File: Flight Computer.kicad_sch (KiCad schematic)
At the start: 28 parts, among them Q1 MMBT2222A, U6 STM32L476VETx, Y1 16MHz

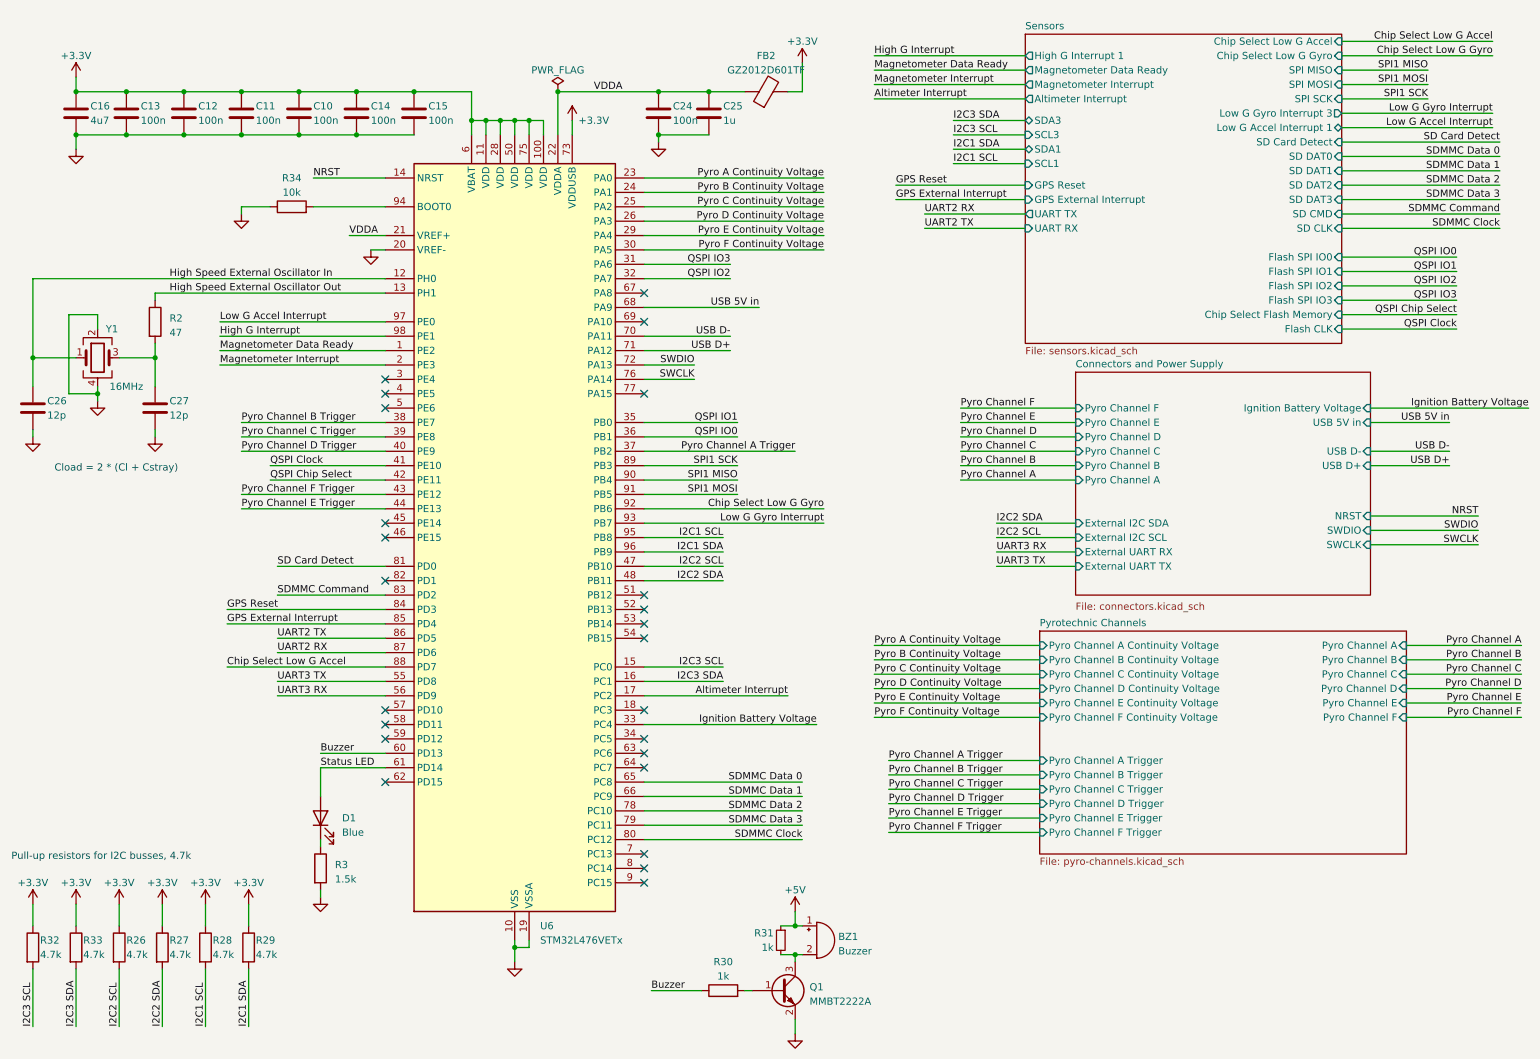
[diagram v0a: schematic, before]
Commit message: How many sheets do you want? Yes
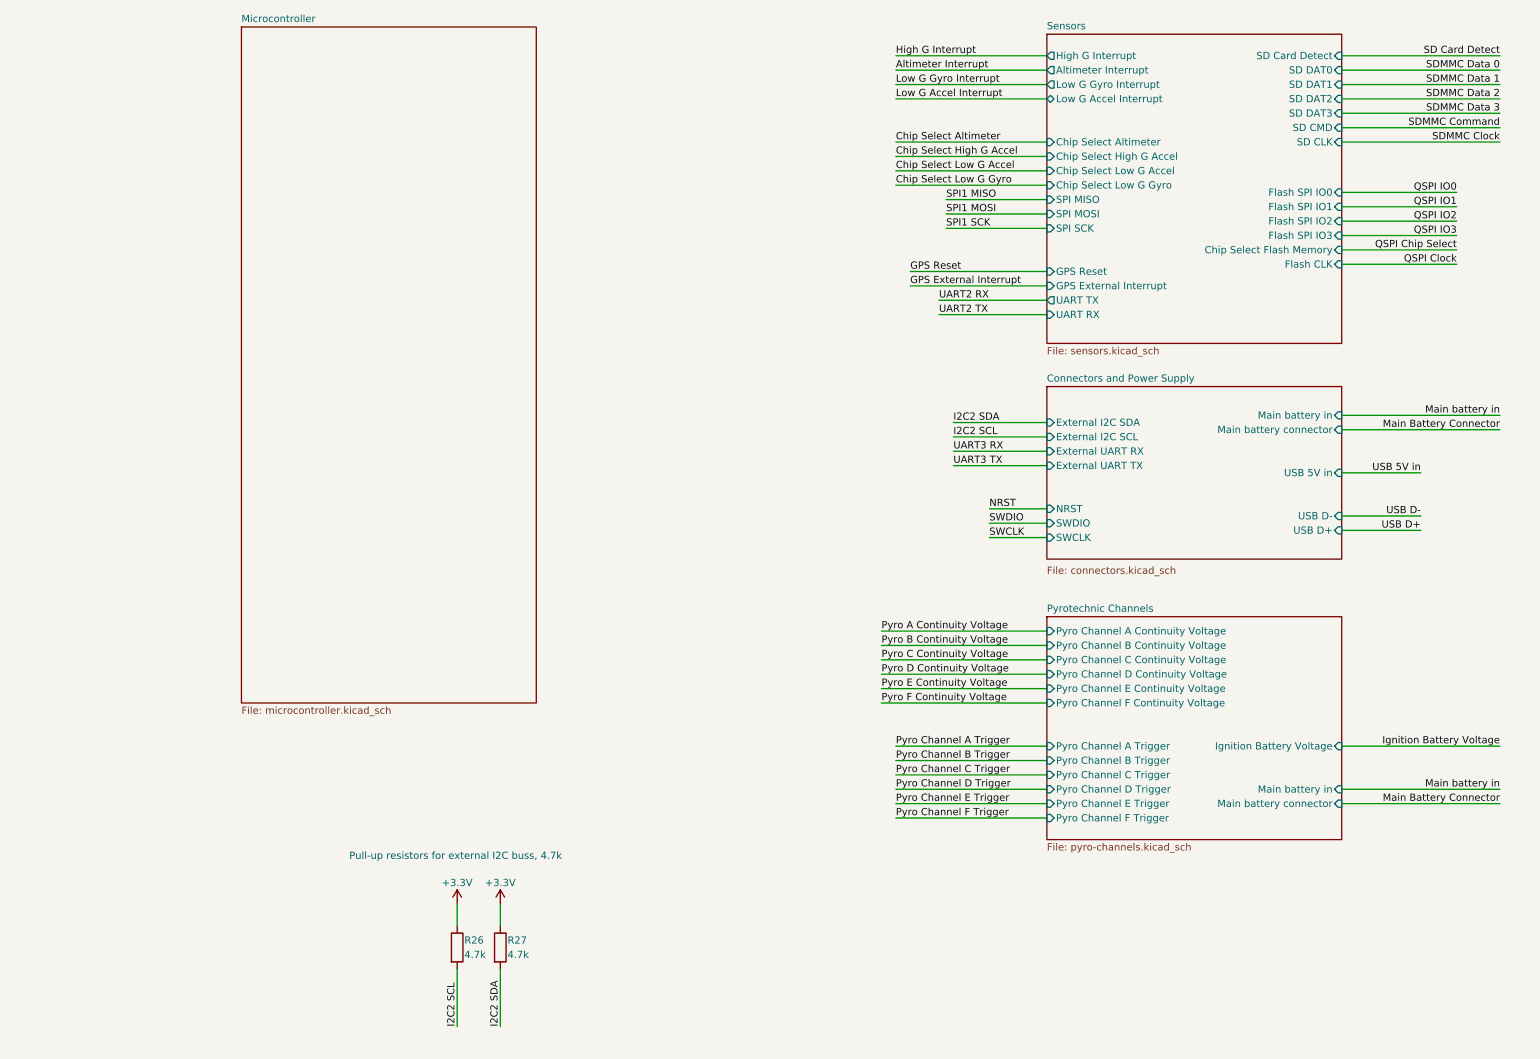
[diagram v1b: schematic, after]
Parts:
- removed BZ1: Buzzer, Buzzer_Beeper:Buzzer_TDK_PS1240P02BT_D12.2mm_H6.5mm, symbol Device:Buzzer
- removed C10, C11, C12, C13, C14, C15, C24: 100n, Capacitor_SMD:C_0402_1005Metric, symbol Device:C
- removed C16: 4u7, Capacitor_SMD:C_0603_1608Metric, symbol Device:C
- removed C25: 1u, Capacitor_SMD:C_0603_1608Metric, symbol Device:C
- removed C26, C27: 12p, Capacitor_SMD:C_0402_1005Metric, symbol Device:C
- removed D1: Blue, LED_SMD:LED_0805_2012Metric, symbol Device:LED
- removed FB2: GZ2012D601TF, Inductor_SMD:L_0805_2012Metric, symbol Device:FerriteBead
- removed Q1: MMBT2222A, Package_TO_SOT_SMD:SOT-23, symbol Transistor_BJT:MMBT3904
- removed R2: 47, Resistor_SMD:R_0603_1608Metric, symbol Device:R
- removed R28, R29, R32, R33: 4.7k, Resistor_SMD:R_0402_1005Metric, symbol Device:R
- removed R3: 1.5k, Resistor_SMD:R_0603_1608Metric, symbol Device:R
- removed R30: 1k, Resistor_SMD:R_0603_1608Metric, symbol Device:R
- removed R31: 1k, Resistor_SMD:R_0603_1608Metric, symbol Device:R_Small
- removed R34: 10k, Resistor_SMD:R_0402_1005Metric, symbol Device:R
- removed U6: STM32L476VETx, Package_QFP:LQFP-100_14x14mm_P0.5mm, symbol MCU_ST_STM32L4:STM32L476VETx
- removed Y1: 16MHz, Crystal:Crystal_SMD_3225-4Pin_3.2x2.5mm, symbol Device:Crystal_GND24
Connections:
- no-connect marks 24 -> 0
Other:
- added sheet Microcontroller (microcontroller.kicad_sch)
- sheet Connectors and Power Supply ports: added Main battery connector, Main battery in; removed Ignition Battery Voltage, Pyro Channel A, Pyro Channel B, Pyro Channel C, Pyro Channel D, Pyro Channel E, Pyro Channel F
- sheet Pyrotechnic Channels ports: added Ignition Battery Voltage, Main battery connector, Main battery in; removed Pyro Channel A, Pyro Channel B, Pyro Channel C, Pyro Channel D, Pyro Channel E, Pyro Channel F
- sheet Sensors ports: added Chip Select Altimeter, Chip Select High G Accel, High G Interrupt, Low G Accel Interrupt, Low G Gyro Interrupt; removed High G Interrupt 1, Low G Accel Interrupt 1, Low G Gyro Interrupt 3, Magnetometer Data Ready, Magnetometer Interrupt, SCL1, SCL3, SDA1, SDA3
- note added: "Pull-up resistors for external I2C buss, 4.7k"
- note removed: "Cload = 2 * (Cl + Cstray)"
- note removed: "Pull-up resistors for I2C busses, 4.7k"
- moved on the sheet: R26, R27
